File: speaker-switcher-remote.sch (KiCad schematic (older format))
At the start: 17 parts, among them M1 arduino-nano, Q1 TIP31C, Q2 TIP31C

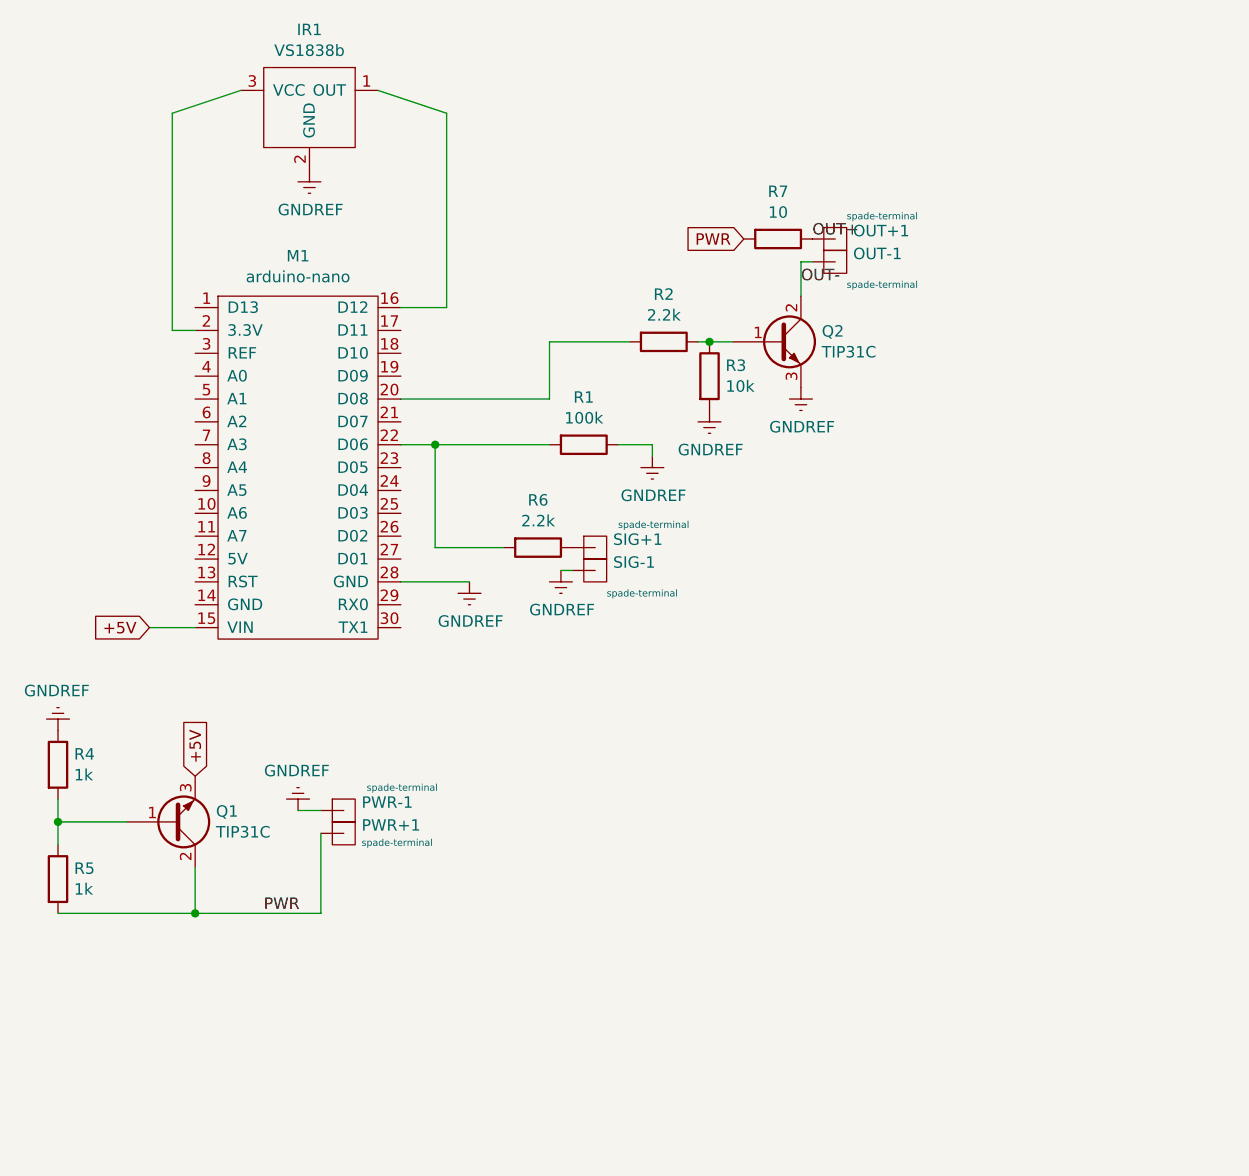
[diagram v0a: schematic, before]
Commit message: Updated with arduino src code
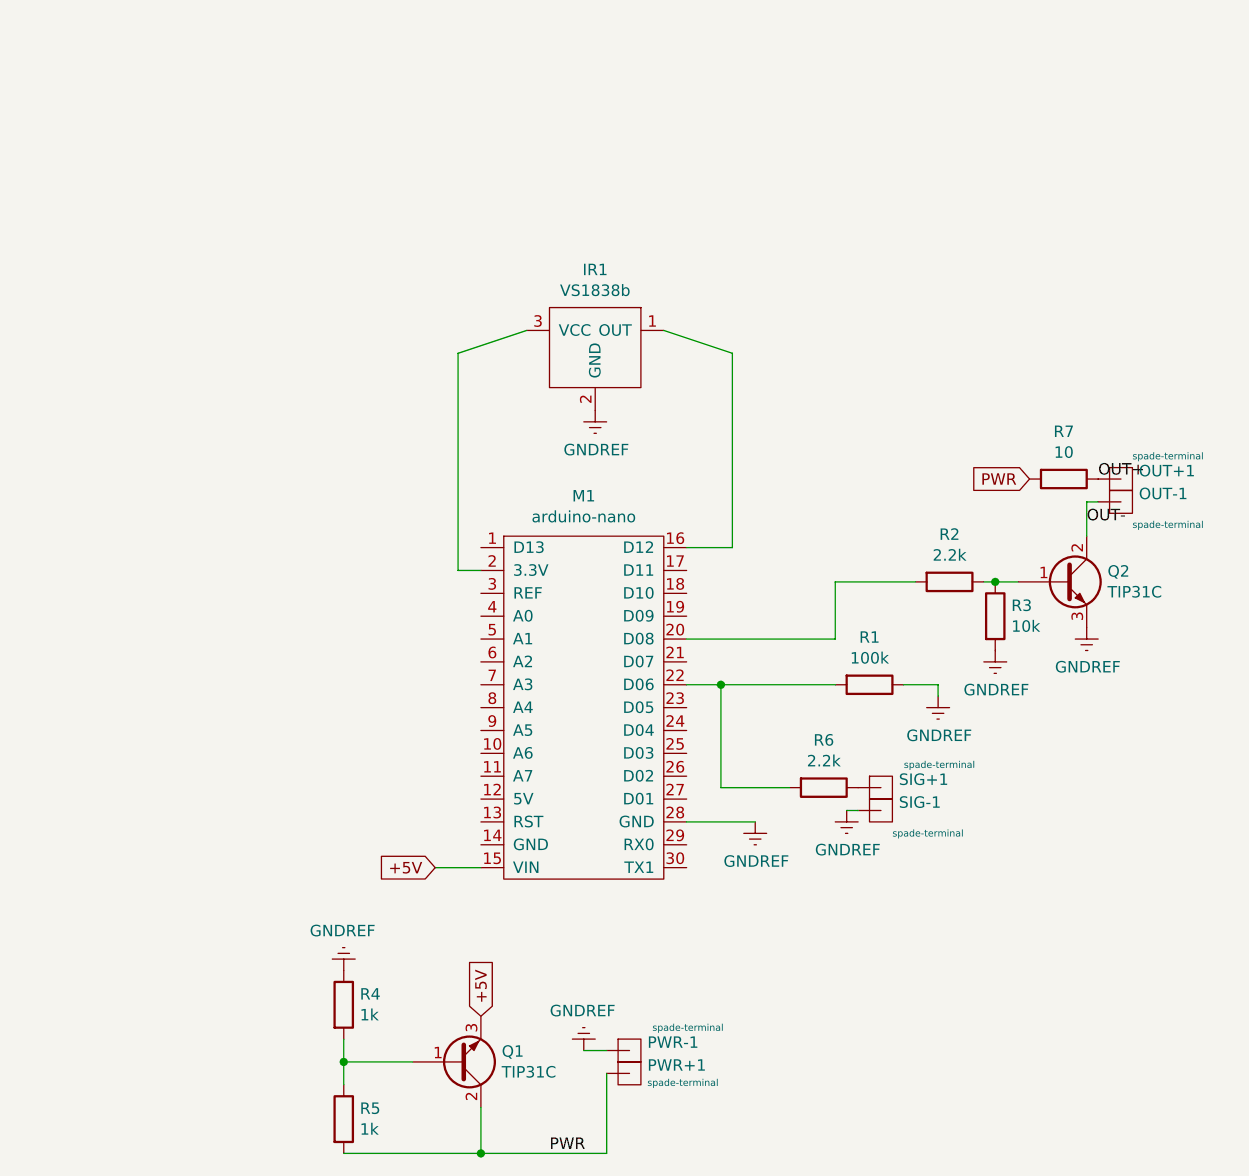
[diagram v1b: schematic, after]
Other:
- moved on the sheet: IR1, M1, OUT+1, OUT-1, PWR+1, PWR-1, Q1, Q2, R1, R2, R3, R4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
